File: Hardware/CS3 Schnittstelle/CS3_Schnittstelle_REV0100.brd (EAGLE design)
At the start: 85 x 65 mm, 18 parts, among them J1 12V, X1 MEBP 8-8G, X2 MEBP 8-8G, X3 MARKLIN-MD-6, X4 MARKLIN-MD-10, X5 MARKLIN-MD-10

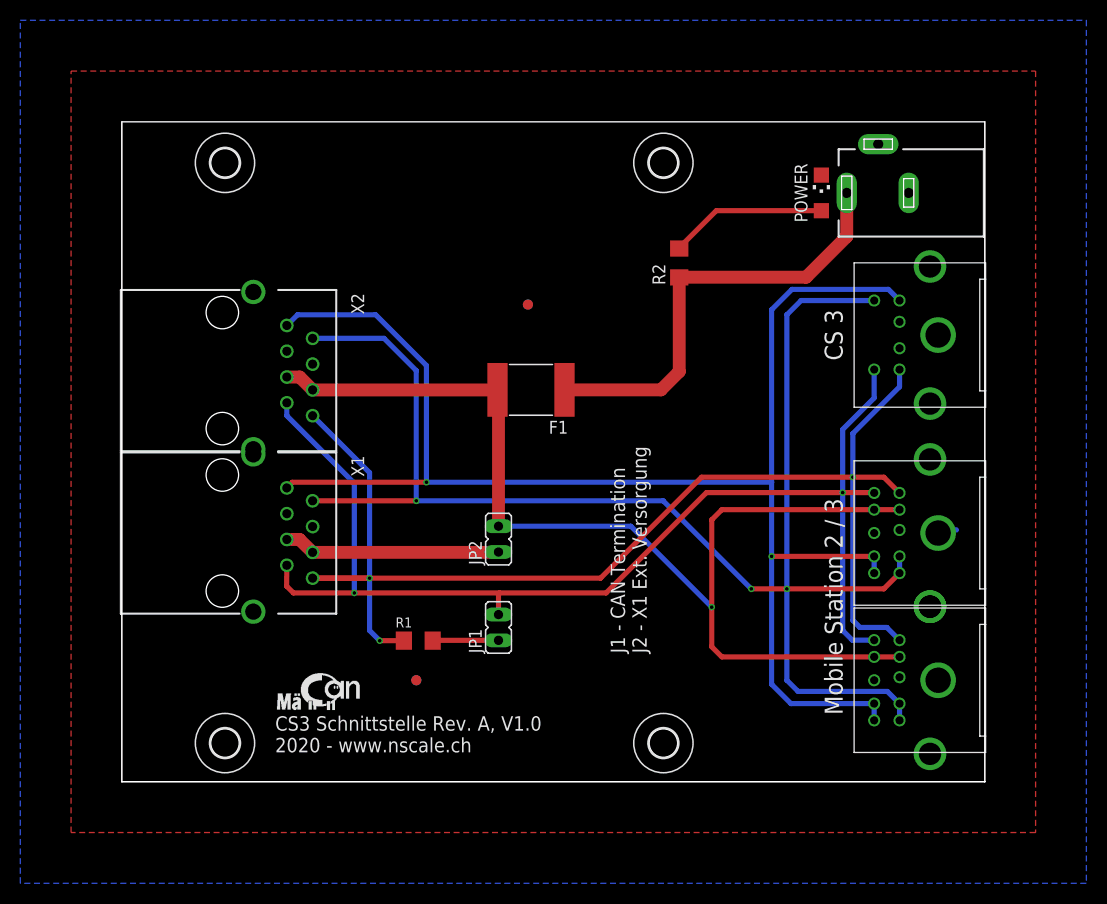
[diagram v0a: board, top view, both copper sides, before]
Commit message: Add files via upload
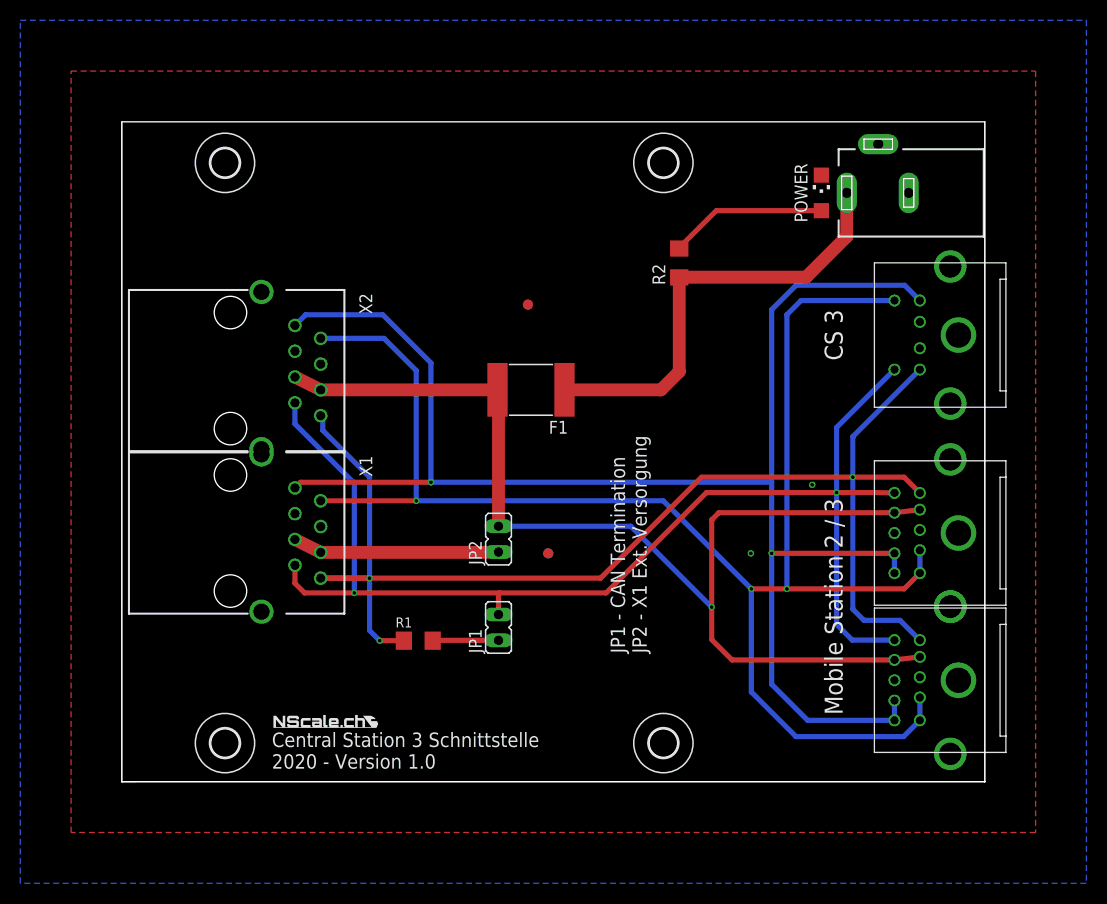
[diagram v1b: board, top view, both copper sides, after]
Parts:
- moved U$2 18.0 mm to (42.0, 22.5)
- moved X3 2.00 mm to (80.6, 44.0)
- moved X4 2.00 mm to (80.6, 10.0)
- moved X5 2.00 mm to (80.6, 24.5)
- moved X1 0.80 mm to (10.7, 24.5)
- moved X2 0.80 mm to (10.7, 40.5)
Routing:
- net GSO: track 146.9 -> 158.7 mm
- net GSB: track 150.8 -> 157.4 mm
- net CANL: track 118.4 -> 122.4 mm
- net VCC_R: track 109.4 -> 112.0 mm
- net CANH: track 127.5 -> 129.7 mm
- net N$1: track 21.4 -> 20.4 mm
- net GND: track 0.05 -> 0.00 mm, vias 0 -> 2
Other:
- board text added: "C:/Users/Patrik Laube/Pictures/logo_sw.bmp"
- board text added: "Central Station 3 Schnittstelle 2020 - Version 1.0"
- board text added: "JP1 - CAN Termination JP2 - X1 Ext. Versorgung"
- board text removed: "CS3 Schnittstelle Rev. A, V1.0 2020 - www.nscale.ch"
- board text removed: "J1 - CAN Termination J2 - X1 Ext. Versorgung"
